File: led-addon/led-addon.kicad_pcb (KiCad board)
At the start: 2 copper layers, 25 x 18 mm, 19 parts, among them J1 VCC, J2 LED+, J3 LED-, J4 PWM, J5 STRT1, J6 GND, J8 STRT2, U1 PAM2804

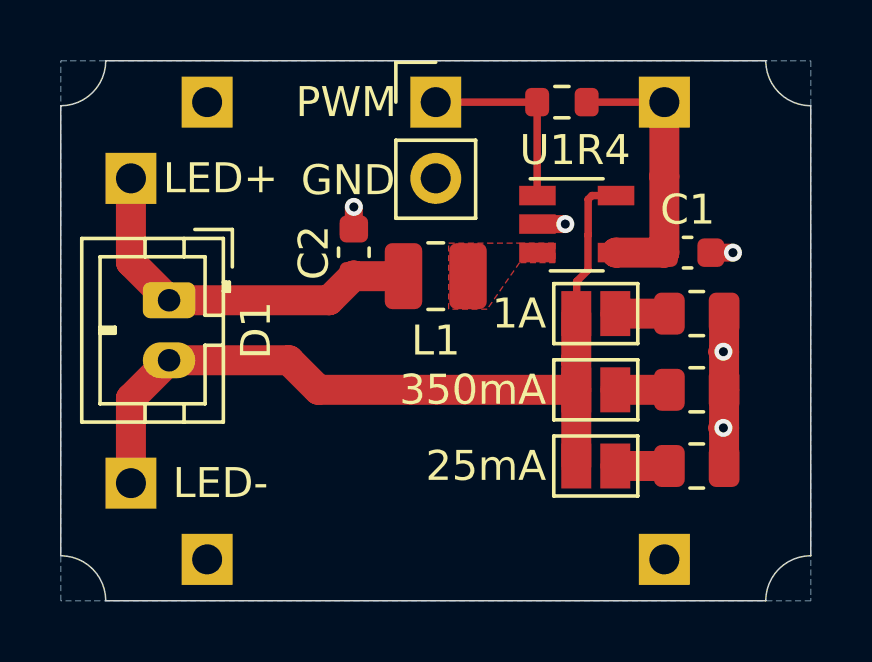
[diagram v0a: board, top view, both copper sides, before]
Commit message: WIP
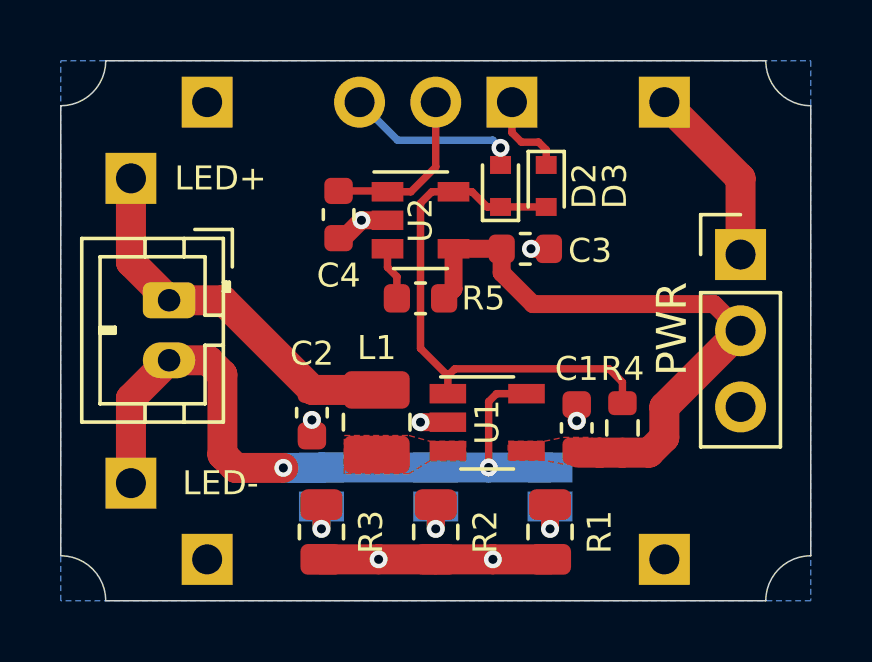
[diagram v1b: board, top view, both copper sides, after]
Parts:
- removed J4: PWM, Connector_PinHeader_2.54mm:PinHeader_1x02_P2.54mm_Vertical
- added C3: 100n, Capacitor_SMD:C_0603_1608Metric, F.Cu at (36.0, 30.3)
- added C4: 100n, Capacitor_SMD:C_0603_1608Metric, F.Cu at (29.8, 29.1)
- added D2: , Diode_SMD:D_SOD-523, F.Cu at (35.2, 28.2)
- added D3: , Diode_SMD:D_SOD-523, F.Cu at (36.7, 28.2)
- added R5: 100k, Resistor_SMD:R_0603_1608Metric, F.Cu at (32.5, 31.9)
- added RV1: 10k, Connector_PinHeader_2.54mm:PinHeader_1x03_P2.54mm_Vertical, B.Cu at (35.6, 25.4)
- added SW1: PWR, Connector_PinHeader_2.54mm:PinHeader_1x03_P2.54mm_Vertical, F.Cu at (43.2, 30.5)
- added U2: MIC1557, Package_TO_SOT_SMD:SOT-23-5, F.Cu at (32.5, 29.3)
- JP1, JP2, JP3: moved to B.Cu
- moved R3 12.7 mm to (29.2, 39.7), turned to 270 degrees
- moved R4 11.0 mm to (39.2, 36.3), turned to 90 degrees
- moved R2 9.91 mm to (33.0, 39.7), turned to 270 degrees
- moved JP3 9.17 mm to (29.2, 38.2), turned to 270 degrees
- moved R1 8.77 mm to (36.8, 39.7), turned to 270 degrees
- moved U1 7.25 mm to (34.7, 36.1)
- moved C1 6.91 mm to (37.7, 36.3), turned to 90 degrees
- moved JP2 6.24 mm to (33.0, 38.2), turned to 270 degrees
- moved JP1 5.98 mm to (36.8, 38.2), turned to 270 degrees
- moved C2 5.53 mm to (28.9, 35.8), turned to 270 degrees
- moved L1 5.25 mm to (31.1, 36.1), turned to 270 degrees
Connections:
- J1 pad 1: VCC -> Net-(J1-Pad1)
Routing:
- net Net-(D2-Pad1): track 6.50 -> 18.1 mm
- net VCC: track 9.58 -> 20.6 mm
- net Net-(J1-Pad1): track 0.00 -> 6.13 mm
- net Net-(D2-Pad2): track 0.00 -> 5.90 mm, vias 0 -> 1
- net Net-(C4-Pad1): track 0.00 -> 5.75 mm
- net GND: track 7.52 -> 12.1 mm, vias 5 -> 7
- net Net-(D1-Pad2): track 28.3 -> 23.9 mm, vias 0 -> 2
- net Net-(D3-Pad1): track 0.00 -> 2.90 mm
- net Net-(R5-Pad2): track 0.00 -> 1.78 mm
- net Net-(JP3-Pad2): track 1.70 -> 1.56 mm, vias 0 -> 1
- net Net-(JP2-Pad2): track 1.70 -> 1.56 mm, vias 0 -> 1
- net Net-(JP1-Pad2): track 1.70 -> 1.56 mm, vias 0 -> 1
- added copper zone on F.Cu, net VCC
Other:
- board text added: "CC LED Driver Thomas Bytheway Rev1 ghub: harkonenbade/batt 2021-09-11"
- board text removed: "GND"
- board text removed: "LED Driver CC 25mA-1A Thomas Bytheway Rev1 github: harkonenbade/batt 2021-09-11"
